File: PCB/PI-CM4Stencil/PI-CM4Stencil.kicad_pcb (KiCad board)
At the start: 2 copper layers, 40.2 x 55.2 mm, 1 part

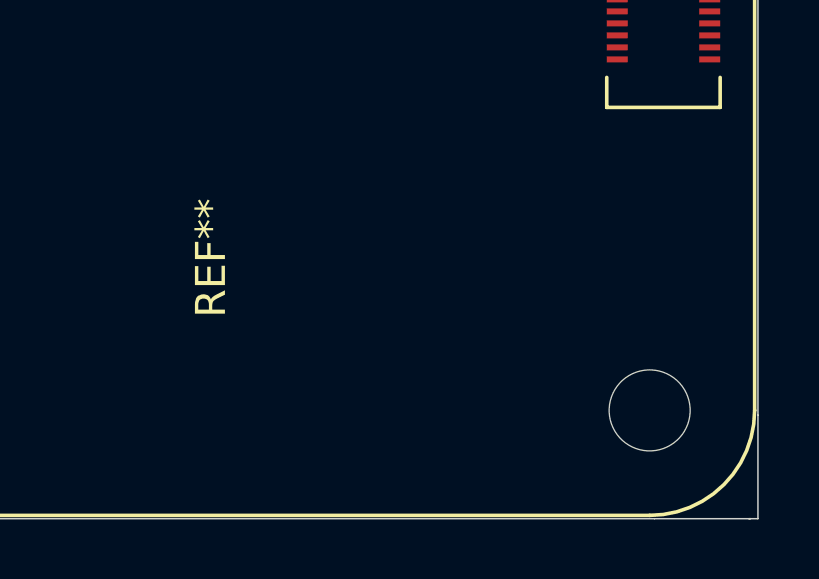
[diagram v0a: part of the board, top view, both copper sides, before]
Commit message: Created gerber files
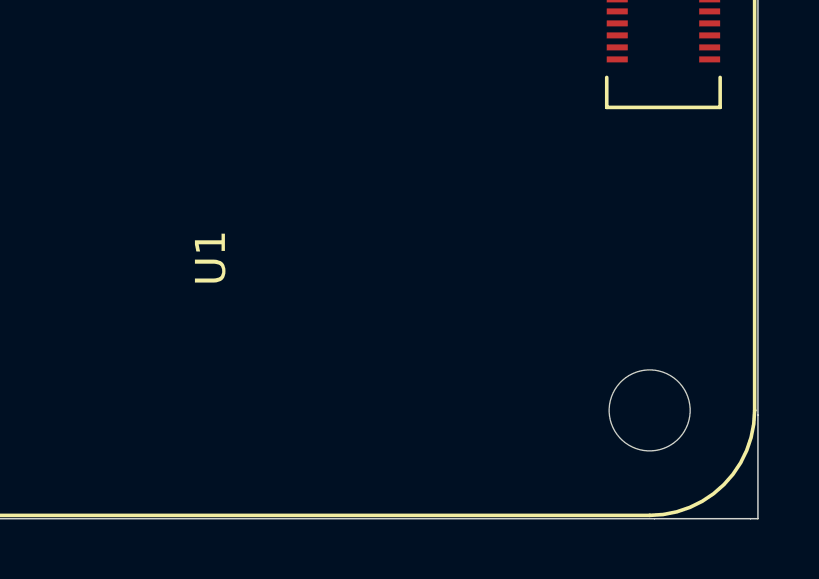
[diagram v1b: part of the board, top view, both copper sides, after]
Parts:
- removed REF**: Raspberry-Pi-4-Compute-Module, PI-CM4Stencil:Pi_CM4
- added U1: Pi_CM4, PI-CM4Stencil:Pi_CM4, F.Cu at (148.6, 97.8)
